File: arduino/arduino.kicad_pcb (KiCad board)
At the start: 2 copper layers, 45.7 x 45.7 mm, 17 parts, among them IC1 ATMEGA328P-P, P1 CONN_6, P2 CONN_2, P3 CONN_6, P4 CONN_6, P5 CONN_1, P6 CONN_6, P7 battery, Q1 16MHz, U1 RFM12B

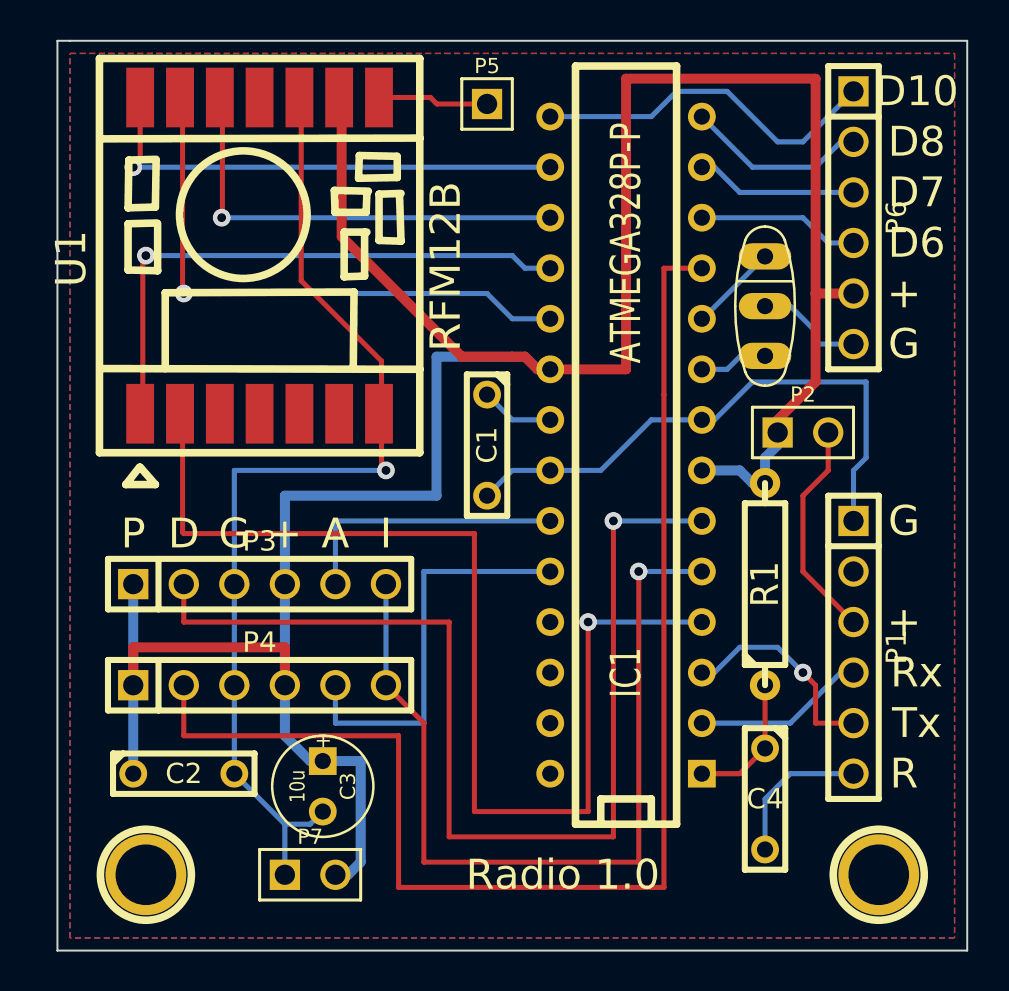
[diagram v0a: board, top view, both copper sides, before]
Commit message: fix port labels
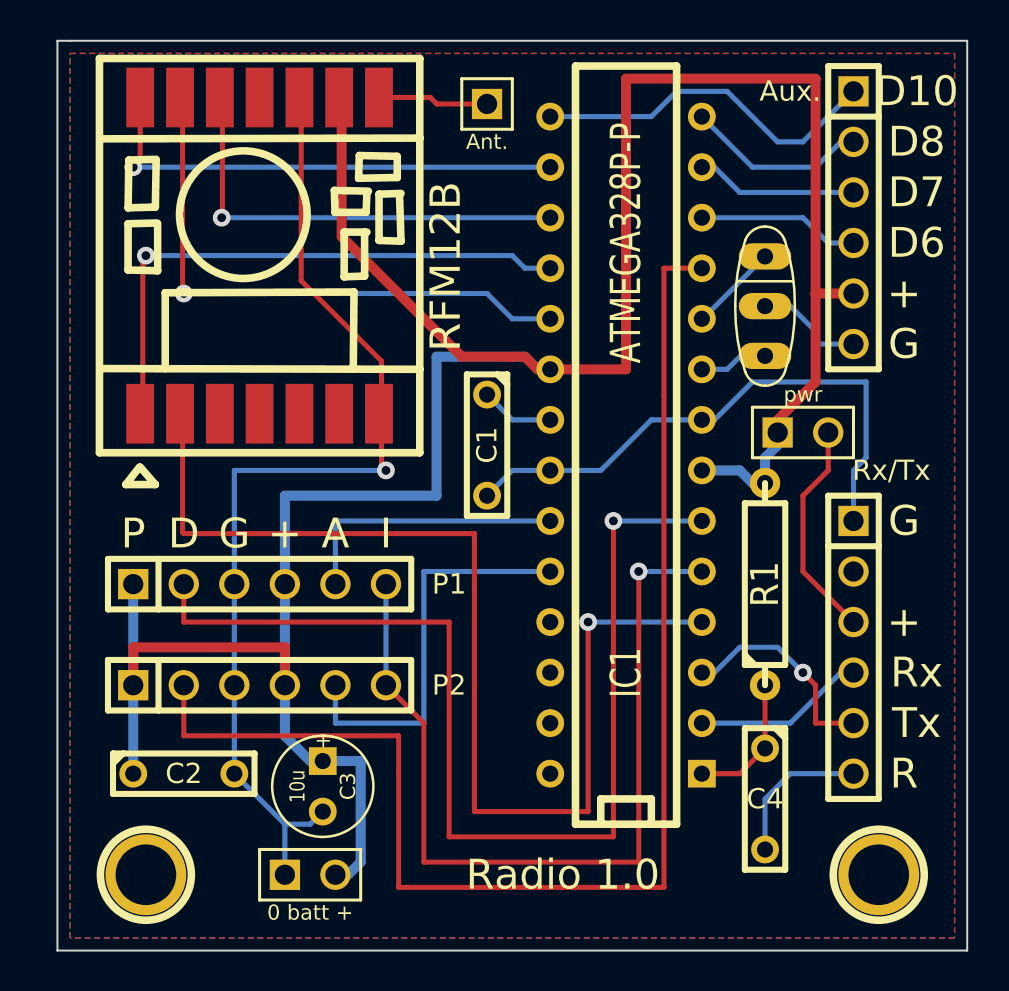
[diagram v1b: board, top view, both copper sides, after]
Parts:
- 0 batt +: renamed from P7
- renumbered U1 to ?, P5 to Ant., P6 to Aux., P3 to P1, P4 to P2, P1 to Rx/Tx, P2 to pwr
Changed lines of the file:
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@@
   (module SMD-RFM12B (layer F.Cu)
     (at 81.28 123.19 270)
-    (fp_text reference U1 (at 0.1524 9.46912 270) (layer F.SilkS)
+    (fp_text reference "" (at 0.1524 9.46912 270) (layer F.SilkS)
       (effects (font (size 1.524 1.524) (thickness 0.3048)))
     )
@@
     (descr "Connecteurs 2 pins")
     (tags "CONN DEV")
-    (fp_text reference P7 (at 0 -1.905) (layer F.SilkS)
+    (fp_text reference "0 batt +" (at 0 1.905) (layer F.SilkS)
       (effects (font (size 0.762 0.762) (thickness 0.1524)))
     )
@@
     (descr "1 pin")
     (tags "CONN DEV")
-    (fp_text reference P5 (at 0 -1.905) (layer F.SilkS)
+    (fp_text reference Ant. (at 0 1.905) (layer F.SilkS)
       (effects (font (size 0.762 0.762) (thickness 0.1524)))
     )
@@
     (descr "Connecteur 6 pins")
     (tags "CONN DEV")
-    (fp_text reference P3 (at 0 -2.159) (layer F.SilkS)
+    (fp_text reference P1 (at 9.525 0) (layer F.SilkS)
       (effects (font (size 1.016 1.016) (thickness 0.2032)))
     )
@@
     (descr "Connecteur 6 pins")
     (tags "CONN DEV")
-    (fp_text reference P4 (at 0 -2.159) (layer F.SilkS)
+    (fp_text reference P2 (at 9.525 0) (layer F.SilkS)
       (effects (font (size 1.016 1.016) (thickness 0.2032)))
     )
@@
     (descr "Connecteur 6 pins")
     (tags "CONN DEV")
-    (fp_text reference P6 (at 0 -2.159 270) (layer F.SilkS)
+    (fp_text reference Aux. (at -6.35 3.175 360) (layer F.SilkS)
       (effects (font (size 1.016 1.016) (thickness 0.2032)))
     )
@@
     (descr "Connecteurs 2 pins")
     (tags "CONN DEV")
-    (fp_text reference P2 (at 0 -1.905) (layer F.SilkS)
+    (fp_text reference pwr (at 0 -1.905) (layer F.SilkS)
       (effects (font (size 0.762 0.762) (thickness 0.1524)))
     )
@@
     (descr "Connecteur 6 pins")
     (tags "CONN DEV")
-    (fp_text reference P1 (at 0 -2.159 270) (layer F.SilkS)
+    (fp_text reference Rx/Tx (at -8.89 -1.905 360) (layer F.SilkS)
       (effects (font (size 1.016 1.016) (thickness 0.2032)))
     )
@@
   (segment (start 79.375 121.285) (end 79.40802 121.25198) (width 0.254) (layer F.Cu) (net 12))
   (via (at 79.375 121.285) (size 0.889) (layers F.Cu B.Cu) (net 12))
-  (segment (start 87.27948 115.24234) (end 89.86266 115.24234) (width 0.254) (layer F.Cu) (net 13) (status 400000))
-  (segment (start 90.19032 115.57) (end 92.71 115.57) (width 0.254) (layer F.Cu) (net 13) (status 800000))
+  (segment (start 87.27948 115.24234) (end 89.86266 115.24234) (width 0.254) (layer F.Cu) (net 13))
+  (segment (start 90.19032 115.57) (end 92.71 115.57) (width 0.254) (layer F.Cu) (net 13))
   (segment (start 89.86266 115.24234) (end 90.19032 115.57) (width 0.254) (layer F.Cu) (net 13))
   (segment (start 103.505 141.605) (end 97.79 141.605) (width 0.254) (layer B.Cu) (net 14))
